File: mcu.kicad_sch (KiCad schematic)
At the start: 41 parts, among them J10 MSD-11-A, J11 Conn_01x04, J5 Conn_01x10, J6 Conn_01x08, J7 USB_C_Receptacle_USB2.0_16P, J8 Conn_01x08, J9 Conn_01x04, U2 ESP32-S3-WROOM-1, U3 STM32C011F4Ux, Y1 Crystal_GND24

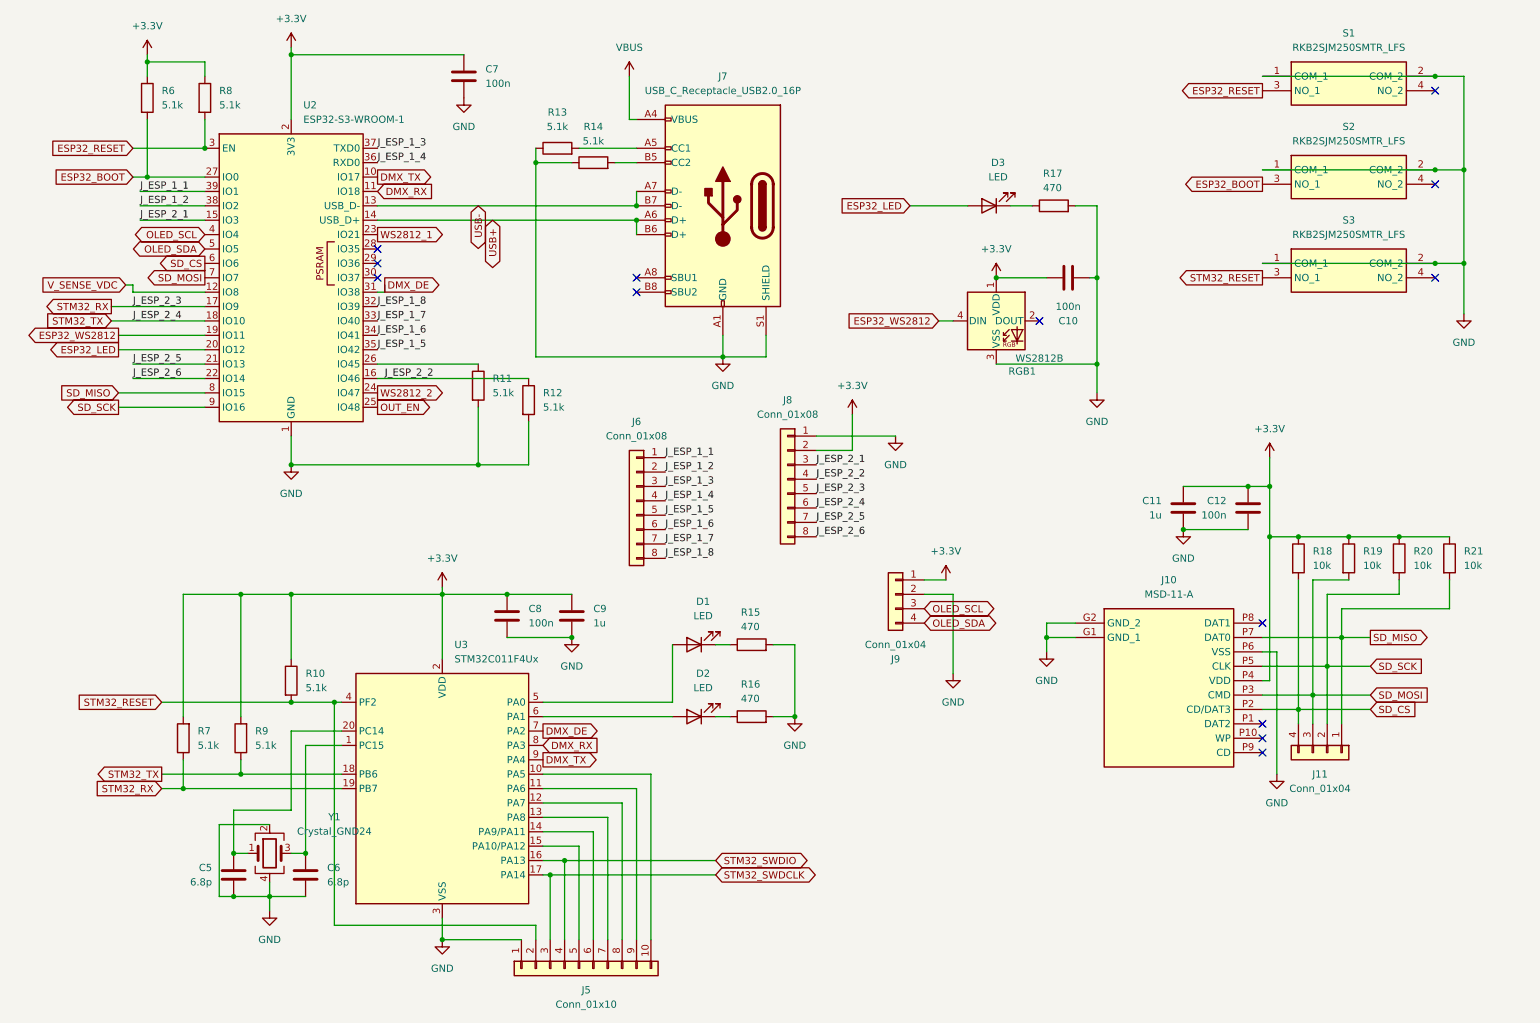
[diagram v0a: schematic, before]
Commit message: complete layout, routing, and silkscreen
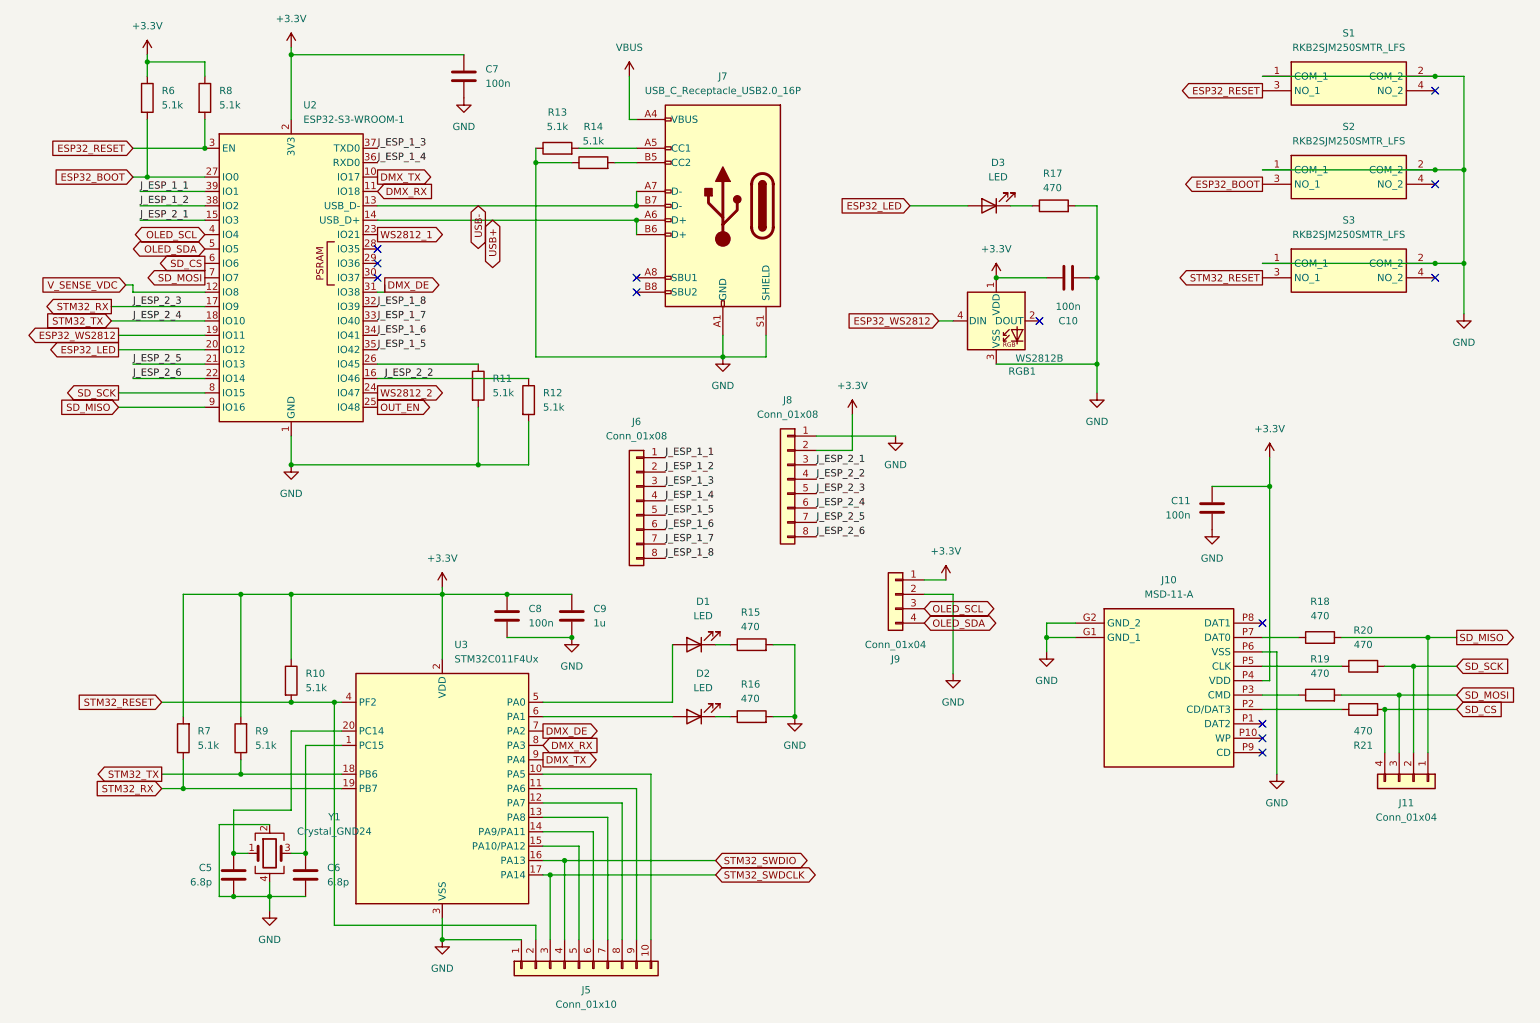
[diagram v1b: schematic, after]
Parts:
- removed C11: 1u, Capacitor_SMD:C_0603_1608Metric_Pad1.08x0.95mm_HandSolder, symbol Device:C
- J6, J8: footprint Connector_PinSocket_2.54mm:PinSocket_1x08_P2.54mm_Vertical -> Connector_PinHeader_2.54mm:PinHeader_1x08_P2.54mm_Vertical
- R18, R19, R20, R21: value 10k -> 470
- renumbered C12 to C11
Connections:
- net +3.3V: no longer R18.1, R19.1, R20.1, R21.1
- net SD_CS: now also R21.2; no longer J10.P2 (CD/DAT3), R18.2
- net SD_MISO: now also R18.2, U2.9 (IO16); no longer J10.P7 (DAT0), R21.2, U2.8 (IO15)
- net SD_MOSI: no longer J10.P3 (CMD)
- net SD_SCK: now also U2.8 (IO15); no longer J10.P5 (CLK), U2.9 (IO16)
- new net: J10.P2 (CD/DAT3), R21.1
- new net: J10.P3 (CMD), R19.1
- new net: J10.P5 (CLK), R20.1
- new net: J10.P7 (DAT0), R18.1
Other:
- moved on the sheet: C11, J11
